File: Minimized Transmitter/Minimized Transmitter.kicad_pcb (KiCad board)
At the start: 2 copper layers, 27.1 x 27.1 mm, 11 parts, among them J1 Conn_01x03_Male, J2 Conn_01x02_Male, J4 Conn_01x05_Male, SW1 SW_Push, U1 LPC824M201JHI33, U2 RFM69HCW

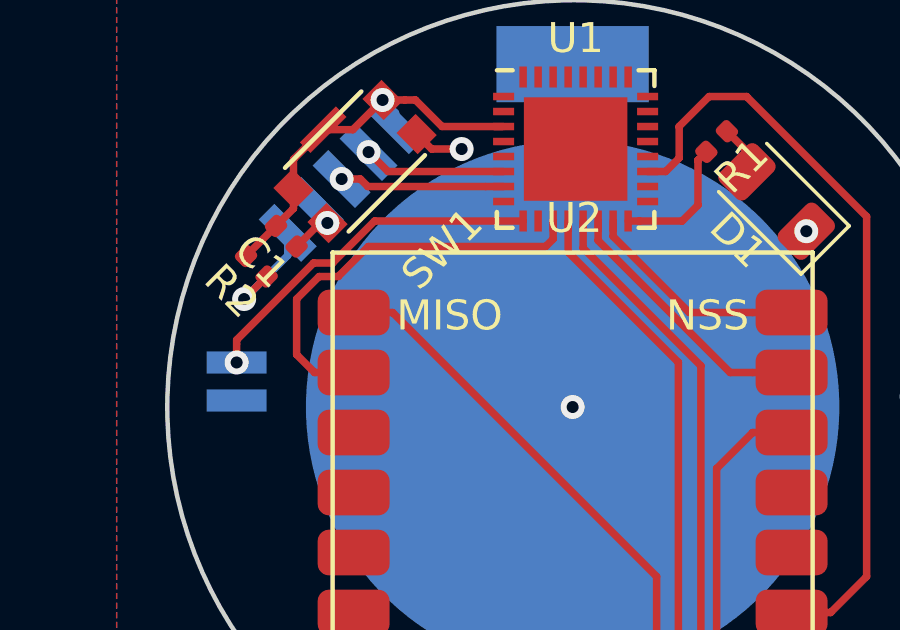
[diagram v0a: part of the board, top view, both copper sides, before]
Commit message: Commit
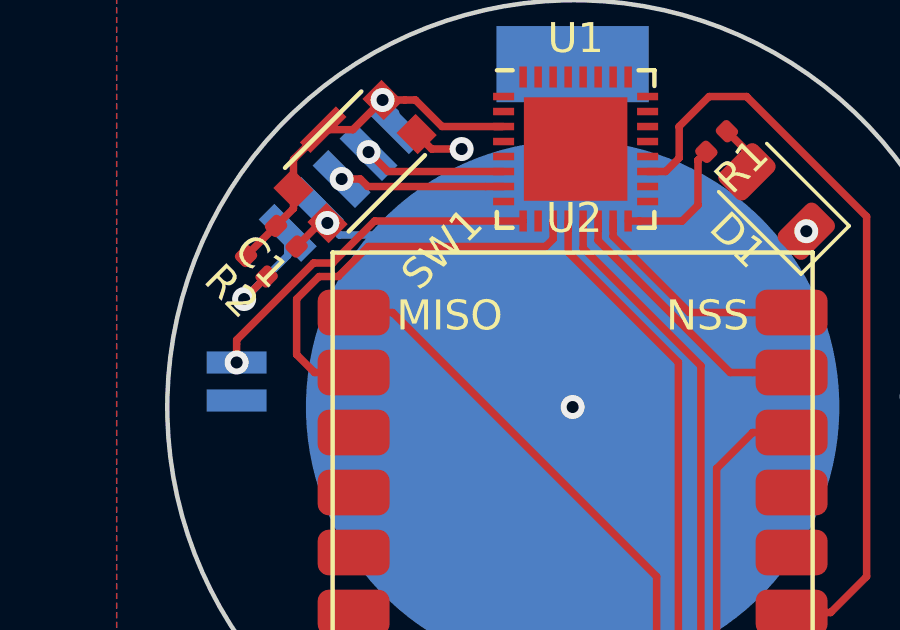
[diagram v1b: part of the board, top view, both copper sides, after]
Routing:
- net GND: track 3.81 -> 14.5 mm
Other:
- board text added: "3v3"
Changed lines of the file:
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@@
-(kicad_pcb (version 20171130) (host pcbnew "(5.0.2)-1")
+(kicad_pcb (version 20171130) (host pcbnew "(5.0.1)-3")
   (general
     (thickness 1.6)
-    (drawings 7)
-    (tracks 101)
+    (drawings 11)
+    (tracks 104)
     (zones 0)
     (modules 11)
@@
     (last_trace_width 0.25)
     (trace_clearance 0.2)
-    (zone_clearance 0.4)
+    (zone_clearance 0.508)
     (zone_45_only no)
     (trace_min 0.2)
@@
       (effects (font (size 0.8 0.8) (thickness 0.12)))
     )
-    (pad 1 smd roundrect (at -1.4 0 135) (size 1.25 1.75) (layers F.Cu F.Paste F.Mask) (roundrect_rratio 0.2)
-      (net 1 GND))
-    (pad 2 smd roundrect (at 1.4 0 135) (size 1.25 1.75) (layers F.Cu F.Paste F.Mask) (roundrect_rratio 0.2)
+    (pad 1 smd roundrect (at -1.399999 0 135) (size 1.25 1.75) (layers F.Cu F.Paste F.Mask) (roundrect_rratio 0.2)
+      (net 1 GND))
+    (pad 2 smd roundrect (at 1.399999 0 135) (size 1.25 1.75) (layers F.Cu F.Paste F.Mask) (roundrect_rratio 0.2)
       (net 36 "Net-(D1-Pad2)"))
     (model ${KISYS3DMOD}/LED_SMD.3dshapes/LED_1206_3216Metric.wrl
@@
     (tags "Surface mounted pin header SMD 2x05 1.27mm double row")
     (attr smd)
-    (fp_text reference J4 (at -1.9 0 225) (layer B.SilkS)
+    (fp_text reference J4 (at 0.141421 -4.525483 225) (layer B.SilkS)
       (effects (font (size 1 1) (thickness 0.15)) (justify mirror))
     )
@@
     (pad 1 smd rect (at 0 2.54 315) (size 2 0.74) (layers B.Cu B.Paste B.Mask)
       (net 2 +3V3))
-    (pad 2 smd rect (at 0 1.27 315) (size 2 0.74) (layers B.Cu B.Paste B.Mask)
+    (pad 2 smd rect (at 0 1.270001 315) (size 2 0.74) (layers B.Cu B.Paste B.Mask)
       (net 1 GND))
     (pad 3 smd rect (at 0 0 315) (size 2 0.74) (layers B.Cu B.Paste B.Mask)
       (net 3 SWDIO))
-    (pad 4 smd rect (at 0 -1.27 315) (size 2 0.74) (layers B.Cu B.Paste B.Mask)
+    (pad 4 smd rect (at 0 -1.270001 315) (size 2 0.74) (layers B.Cu B.Paste B.Mask)
       (net 4 SWDCLK))
     (pad 5 smd rect (at 0 -2.54 315) (size 2 0.74) (layers B.Cu B.Paste B.Mask)
@@
     (tags "Surface mounted pin header SMD 2x05 1.27mm double row")
     (attr smd)
-    (fp_text reference J2 (at -1.9 0 270) (layer B.SilkS)
+    (fp_text reference J2 (at -1.9 0 -90) (layer B.SilkS) hide
       (effects (font (size 1 1) (thickness 0.15)) (justify mirror))
     )
@@
     (pad "" smd rect (at 3.65 1.1 270) (size 1 0.8) (layers F.Cu F.Paste F.Mask))
   )
-  (gr_text IO (at 154.3 68.7) (layer B.SilkS)
+  (gr_text "GND\n" (at 152 78.5) (layer B.SilkS)
+    (effects (font (size 0.6 0.6) (thickness 0.15)) (justify mirror))
+  )
+  (gr_text TX (at 152 75.15) (layer B.SilkS)
+    (effects (font (size 0.6 0.6) (thickness 0.15)) (justify mirror))
+  )
+  (gr_text 3v3 (at 152.75 70.35) (layer B.SilkS)
     (effects (font (size 0.5 0.5) (thickness 0.125)) (justify mirror))
   )
-  (gr_text CLK (at 155.1 67.7) (layer B.SilkS)
+  (gr_text "GND\n" (at 153.6 69.3) (layer B.SilkS)
     (effects (font (size 0.5 0.5) (thickness 0.125)) (justify mirror))
   )
-  (gr_text nR (at 156.1 64.3) (layer B.SilkS)
+  (gr_text IO (at 154.6 68.35) (layer B.SilkS)
+    (effects (font (size 0.5 0.5) (thickness 0.125)) (justify mirror))
+  )
+  (gr_text CLK (at 155.4 67.4) (layer B.SilkS)
+    (effects (font (size 0.5 0.5) (thickness 0.125)) (justify mirror))
+  )
+  (gr_text nR (at 156.9 66.55) (layer B.SilkS)
     (effects (font (size 0.5 0.5) (thickness 0.125)) (justify mirror))
   )
@@
   (via (at 174.5 77.25) (size 0.8) (drill 0.4) (layers F.Cu B.Cu) (net 1))
   (via (at 163.2 77.6) (size 0.8) (drill 0.4) (layers F.Cu B.Cu) (net 1))
+  (segment (start 157.464763 71.864763) (end 163.2 77.6) (width 0.25) (layer B.Cu) (net 1))
+  (segment (start 155.425067 71.864763) (end 157.464763 71.864763) (width 0.25) (layer B.Cu) (net 1))
+  (segment (start 155.025068 71.464764) (end 155.425067 71.864763) (width 0.25) (layer B.Cu) (net 1))
   (via (at 152.25 74) (size 0.8) (drill 0.4) (layers F.Cu B.Cu) (net 2))
   (segment (start 153 73.25) (end 152.25 74) (width 0.25) (layer F.Cu) (net 2))
@@
     (connect_pads (clearance 0.4))
     (min_thickness 0.254)
-    (fill (arc_segments 16) (thermal_gap 0.508) (thermal_bridge_width 0.508))
+    (fill yes (arc_segments 16) (thermal_gap 0.508) (thermal_bridge_width 0.508))
     (polygon
       (pts
@@
   )
   (zone (net 1) (net_name GND) (layer B.Cu) (hatch edge 0.508)
-    (connect_pads yes (clearance 0.508))
+    (connect_pads (clearance 0.508))
     (min_thickness 0.254)
-    (fill (arc_segments 16) (thermal_gap 0.508) (thermal_bridge_width 0.508))
+    (fill yes (arc_segments 16) (thermal_gap 0.508) (thermal_bridge_width 0.508))
     (polygon
       (pts
